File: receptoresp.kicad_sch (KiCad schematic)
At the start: 3 parts

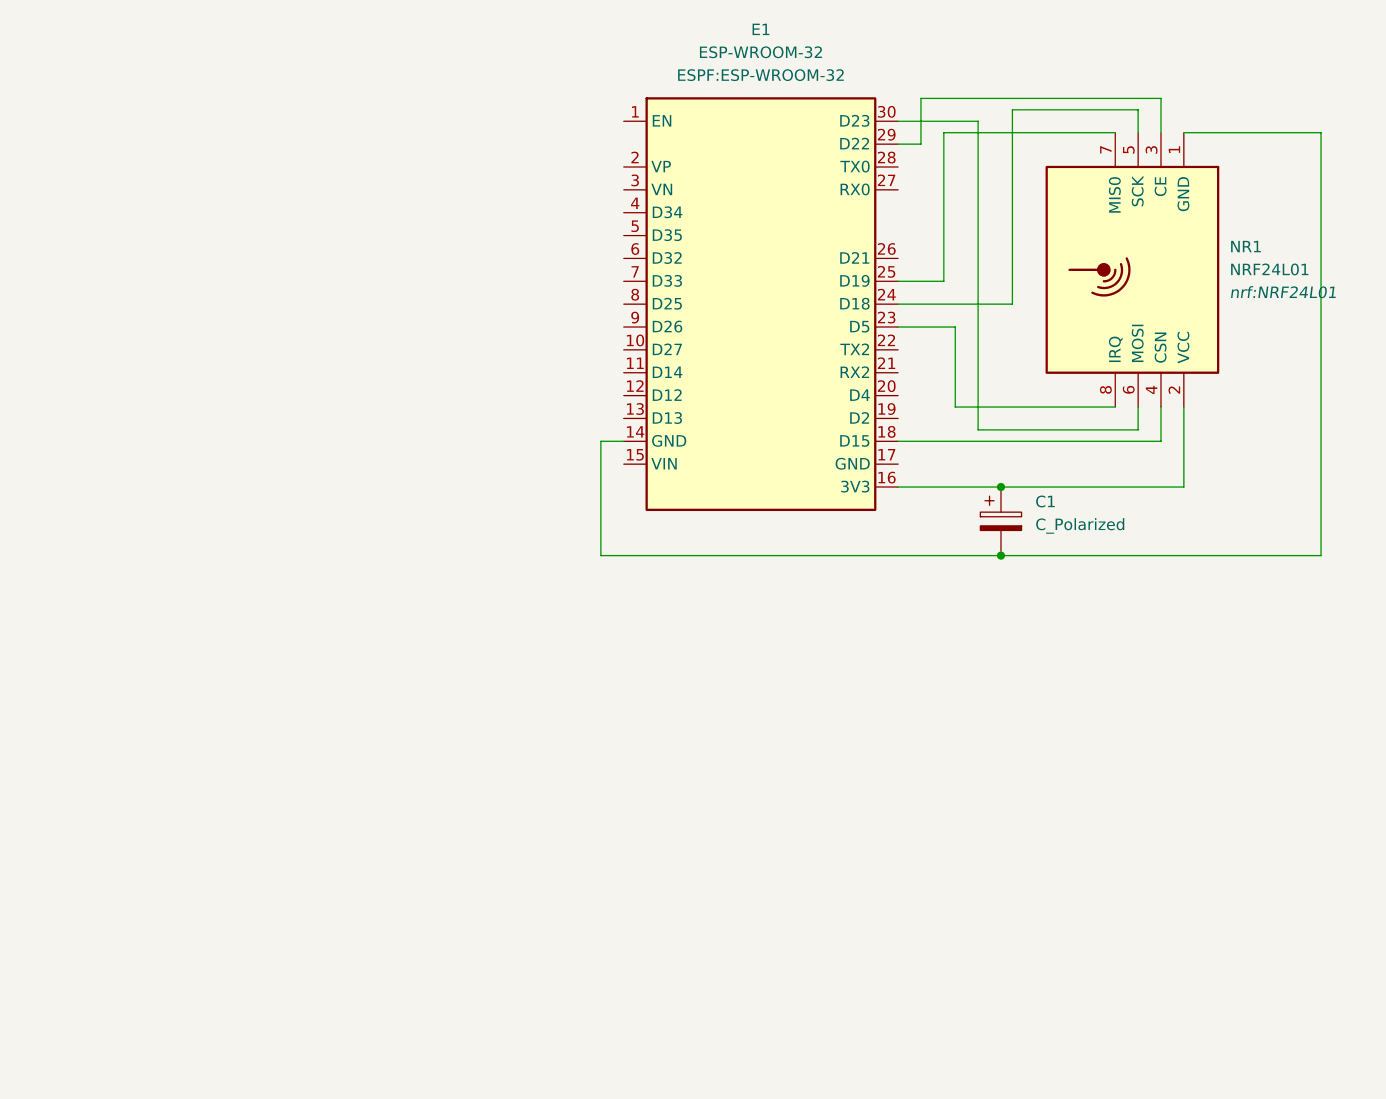
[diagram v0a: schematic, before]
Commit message: pcb pi pico
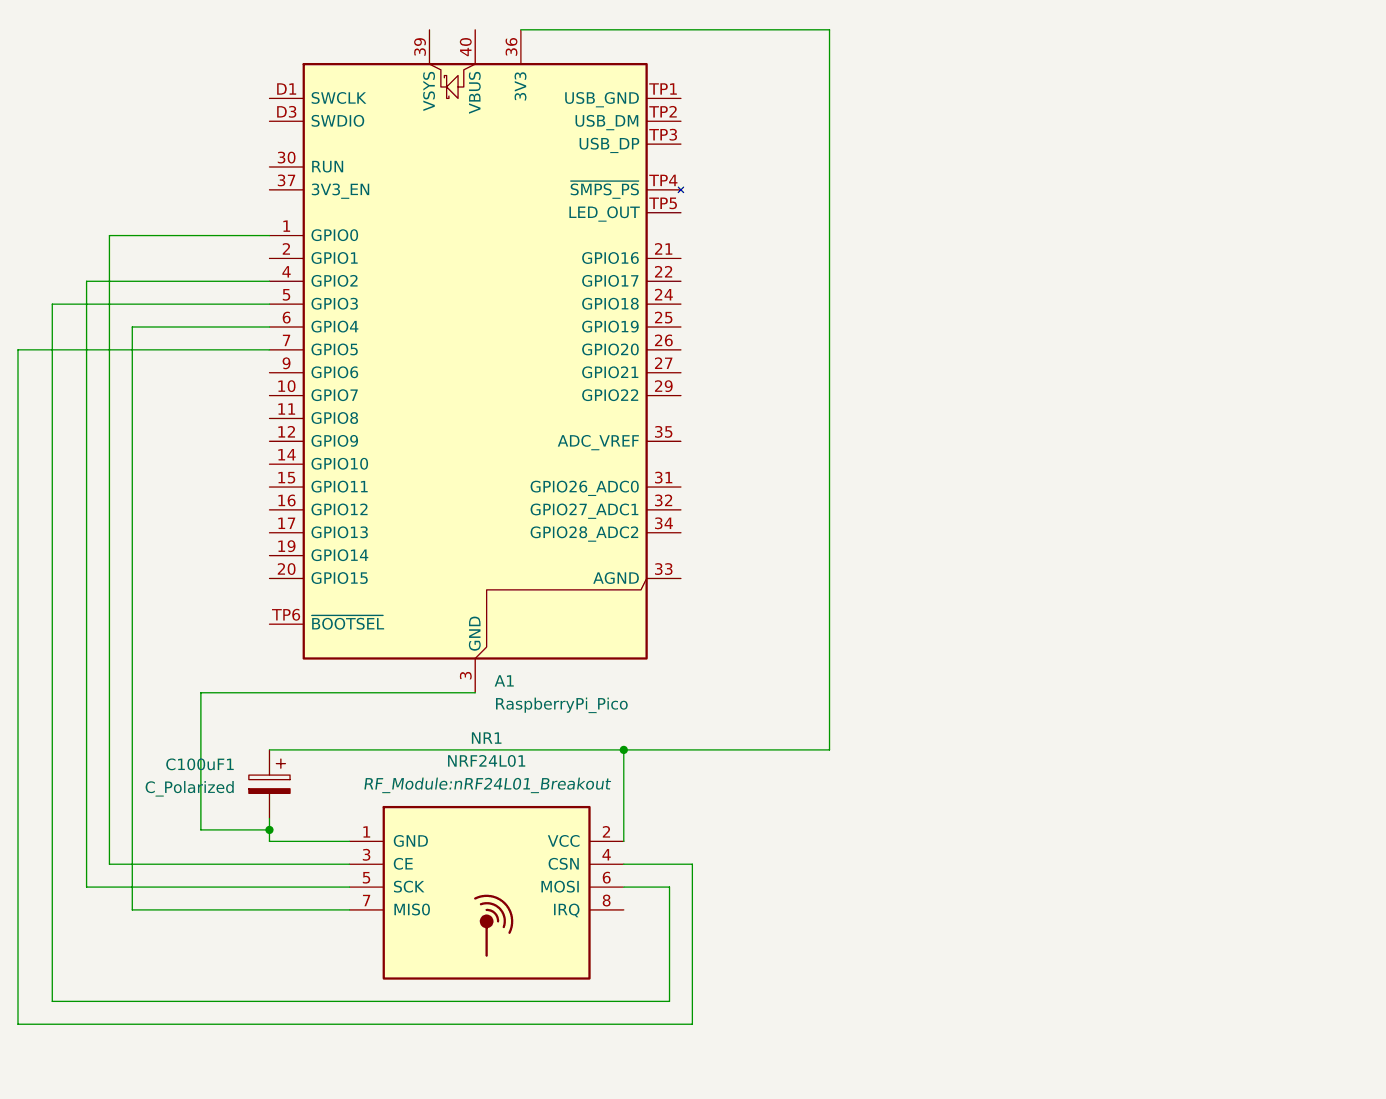
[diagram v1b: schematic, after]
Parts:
- removed C1: C_Polarized, Capacitor_THT:C_Disc_D3.0mm_W1.6mm_P2.50mm, symbol Device:C_Polarized
- removed E1: ESP-WROOM-32, ESPF:ESP-WROOM-32, symbol ESP:ESP-WROOM-32
- added A1: RaspberryPi_Pico, Module:RaspberryPi_Pico_Common_THT, symbol MCU_Module:RaspberryPi_Pico_Extensive
- added C100uF1: C_Polarized, Capacitor_THT:C_Radial_D4.0mm_H5.0mm_P1.50mm, symbol Device:C_Polarized
- NR1: footprint nrf:NRF24L01 -> RF_Module:nRF24L01_Breakout
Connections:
- net at NR1.2 (VCC): now also A1.36 (3V3), C100uF1.1
- net at NR1.1 (GND): now also A1.13 (GND), A1.18 (GND), A1.23 (GND), A1.28 (GND), A1.3 (GND), A1.38 (GND), A1.8 (GND), A1.D2 (GND), C100uF1.2
- net at NR1.3 (CE): now also A1.1 (GPIO0)
- net at NR1.4 (CSN): now also A1.7 (GPIO5)
- net at NR1.5 (SCK): now also A1.4 (GPIO2)
- net at NR1.6 (MOSI): now also A1.5 (GPIO3)
- net at NR1.7 (MIS0): now also A1.6 (GPIO4)
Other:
- moved on the sheet: NR1
